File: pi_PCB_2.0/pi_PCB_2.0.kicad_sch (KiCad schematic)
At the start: 7 parts

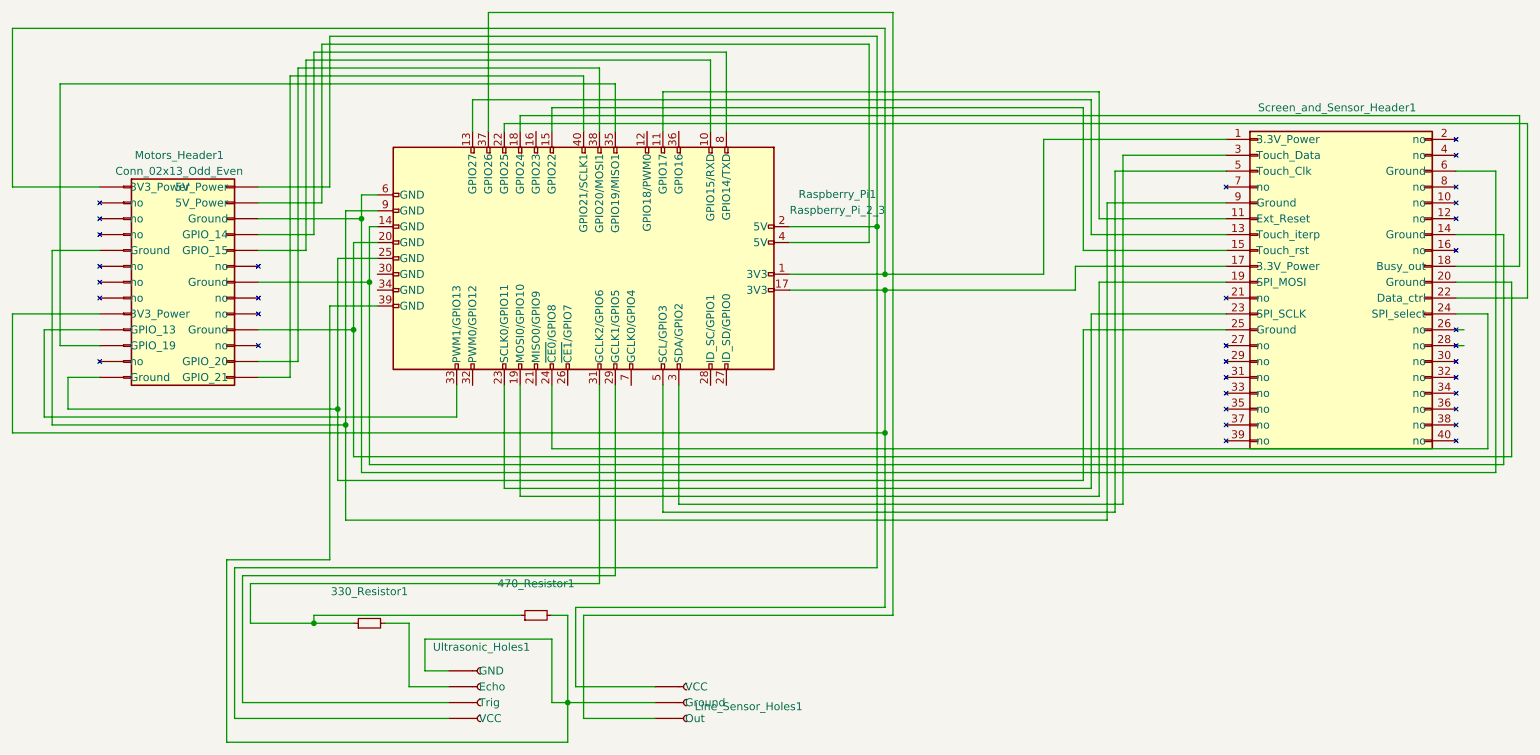
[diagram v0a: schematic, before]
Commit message: PCB Final?
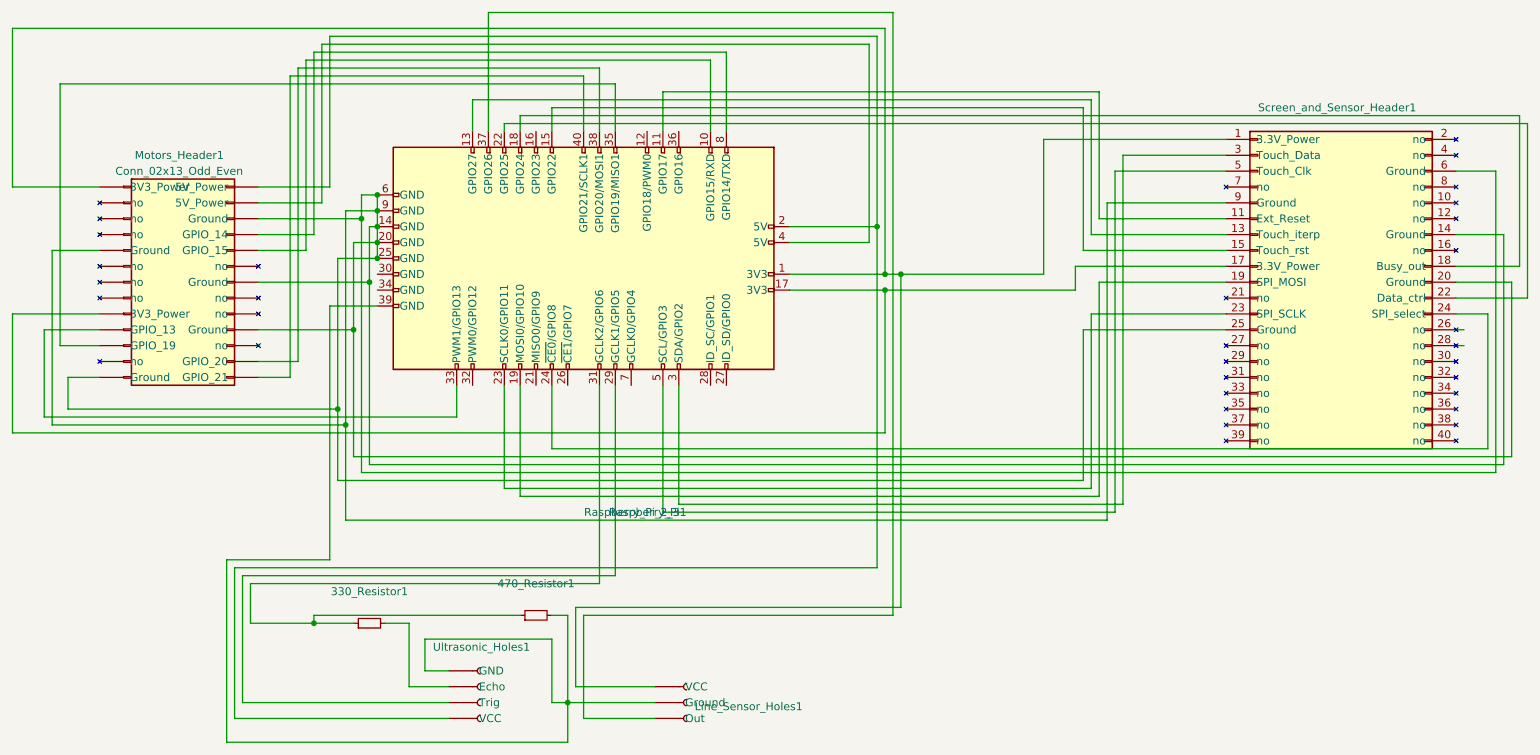
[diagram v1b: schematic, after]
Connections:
- net at Motors_Header1.1 (3V3_Power), Raspberry_Pi1.1 (3V3), Screen_and_Sensor_Header1.1 (3.3V_Power): now also Line_Sensor_Holes1.1 (VCC)
- net at Motors_Header1.14 (Ground), Raspberry_Pi1.14 (GND), Screen_and_Sensor_Header1.14 (Ground): now also Motors_Header1.20 (Ground), Motors_Header1.25 (Ground), Motors_Header1.6 (Ground), Motors_Header1.9 (Ground), Raspberry_Pi1.20 (GND), Raspberry_Pi1.25 (GND), Raspberry_Pi1.6 (GND), Raspberry_Pi1.9 (GND), Screen_and_Sensor_Header1.20 (Ground), Screen_and_Sensor_Header1.25 (Ground), Screen_and_Sensor_Header1.6 (Ground), Screen_and_Sensor_Header1.9 (Ground)
- net at Motors_Header1.17 (3V3_Power), Raspberry_Pi1.17 (3V3), Screen_and_Sensor_Header1.17 (3.3V_Power): no longer Line_Sensor_Holes1.1 (VCC)
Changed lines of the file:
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@@
   (junction (at 163.83 95.25) (diameter 0) (color 0 0 0 0)
   )
+  (junction (at 83.82 92.71) (diameter 0) (color 0 0 0 0)
+  )
   (junction (at 165.1 102.87) (diameter 0) (color 0 0 0 0)
   )
-  (junction (at 165.1 128.27) (diameter 0) (color 0 0 0 0)
-  )
   (junction (at 77.47 124.46) (diameter 0) (color 0 0 0 0)
   )
+  (junction (at 83.82 95.25) (diameter 0) (color 0 0 0 0)
+  )
+  (junction (at 83.82 97.79) (diameter 0) (color 0 0 0 0)
+  )
+  (junction (at 83.82 90.17) (diameter 0) (color 0 0 0 0)
+  )
   (junction (at 82.55 104.14) (diameter 0) (color 0 0 0 0)
   )
@@
   (junction (at 80.01 111.76) (diameter 0) (color 0 0 0 0)
   )
+  (junction (at 83.82 100.33) (diameter 0) (color 0 0 0 0)
+  )
   (junction (at 73.66 158.75) (diameter 0) (color 0 0 0 0)
   )
@@
   (junction (at 78.74 127) (diameter 0) (color 0 0 0 0)
   )
+  (junction (at 167.64 102.87) (diameter 0) (color 0 0 0 0)
+  )
   (junction (at 81.28 93.98) (diameter 0) (color 0 0 0 0)
   )
@@
     (stroke (width 0) (type default))
   )
-  (wire (pts (xy 165.1 128.27) (xy 165.1 156.21))
-    (stroke (width 0) (type default))
-  )
   (wire (pts (xy 82.55 133.35) (xy 82.55 104.14))
     (stroke (width 0) (type default))
@@
     (stroke (width 0) (type default))
   )
-  (wire (pts (xy 115.57 156.21) (xy 165.1 156.21))
-    (stroke (width 0) (type default))
-  )
   (wire (pts (xy 137.16 68.58) (xy 72.39 68.58))
     (stroke (width 0) (type default))
   )
+  (wire (pts (xy 83.82 92.71) (xy 83.82 95.25))
+    (stroke (width 0) (type default))
+  )
   (wire (pts (xy 31.75 127) (xy 31.75 99.06))
     (stroke (width 0) (type default))
@@
     (stroke (width 0) (type default))
   )
-  (wire (pts (xy 190.5 102.87) (xy 165.1 102.87))
+  (wire (pts (xy 190.5 102.87) (xy 167.64 102.87))
     (stroke (width 0) (type default))
   )
@@
     (stroke (width 0) (type default))
   )
+  (wire (pts (xy 115.57 156.21) (xy 167.64 156.21))
+    (stroke (width 0) (type default))
+  )
   (wire (pts (xy 63.5 158.75) (xy 73.66 158.75))
     (stroke (width 0) (type default))
@@
     (stroke (width 0) (type default))
   )
-  (wire (pts (xy 82.55 104.14) (xy 82.55 95.25))
+  (wire (pts (xy 82.55 95.25) (xy 82.55 104.14))
     (stroke (width 0) (type default))
   )
@@
     (stroke (width 0) (type default))
   )
+  (wire (pts (xy 83.82 95.25) (xy 83.82 97.79))
+    (stroke (width 0) (type default))
+  )
   (wire (pts (xy 104.14 78.74) (xy 104.14 80.01))
     (stroke (width 0) (type default))
@@
     (stroke (width 0) (type default))
   )
+  (wire (pts (xy 167.64 102.87) (xy 167.64 156.21))
+    (stroke (width 0) (type default))
+  )
+  (wire (pts (xy 167.64 102.87) (xy 165.1 102.87))
+    (stroke (width 0) (type default))
+  )
   (wire (pts (xy 256.54 96.52) (xy 264.16 96.52))
     (stroke (width 0) (type default))
@@
     (stroke (width 0) (type default))
   )
+  (wire (pts (xy 83.82 90.17) (xy 83.82 92.71))
+    (stroke (width 0) (type default))
+  )
   (wire (pts (xy 201.93 140.97) (xy 129.54 140.97))
     (stroke (width 0) (type default))
@@
   )
   (wire (pts (xy 69.85 71.12) (xy 69.85 119.38))
+    (stroke (width 0) (type default))
+  )
+  (wire (pts (xy 83.82 97.79) (xy 83.82 100.33))
     (stroke (width 0) (type default))
   )
@@
   (symbol (lib_id "Connector:Raspberry_Pi_2_3") (at 116.84 100.33 270) (unit 1)
     (in_bom yes) (on_board yes) (dnp no) (fields_autoplaced)
-    (property "Reference" "Raspberry_Pi1" (at 157.48 90.0683 90)
+    (property "Reference" "Raspberry_Pi1" (at 127.1017 140.97 90)
       (effects (font (size 1.27 1.27)))
     )
-    (property "Value" "Raspberry_Pi_2_3" (at 157.48 92.6083 90)
+    (property "Value" "Raspberry_Pi_2_3" (at 124.5617 140.97 90)
       (effects (font (size 1.27 1.27)))
     )

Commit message: Final 3
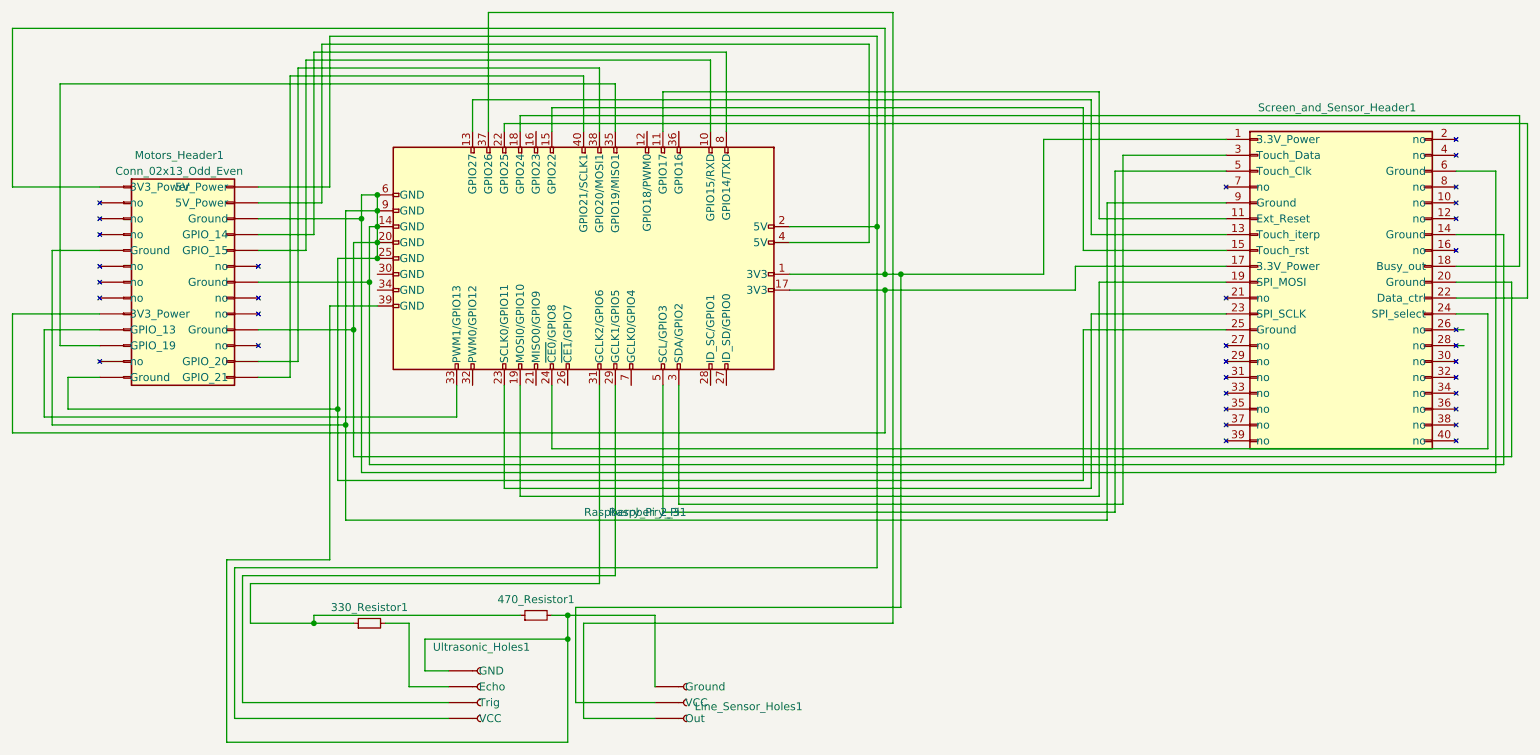
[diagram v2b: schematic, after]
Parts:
- 330_Resistor1, 470_Resistor1: footprint Resistor_THT:R_Axial_DIN0204_L3.6mm_D1.6mm_P1.90mm_Vertical -> Resistor_THT:R_Axial_DIN0207_L6.3mm_D2.5mm_P10.16mm_Horizontal
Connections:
- net at Motors_Header1.1 (3V3_Power), Raspberry_Pi1.1 (3V3), Screen_and_Sensor_Header1.1 (3.3V_Power): now also Line_Sensor_Holes1.2 (VCC); no longer Line_Sensor_Holes1.1 (VCC)
- net at 470_Resistor1.2, Raspberry_Pi1.39 (GND), Ultrasonic_Holes1.1 (GND): now also Line_Sensor_Holes1.1 (Ground); no longer Line_Sensor_Holes1.2 (Ground)
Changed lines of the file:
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@@
 (kicad_sch (version 20230121) (generator eeschema)
   (paper "A4")
+  (junction (at 114.3 157.48) (diameter 0) (color 0 0 0 0)
+  )
   (junction (at 163.83 95.25) (diameter 0) (color 0 0 0 0)
   )
@@
   (junction (at 80.01 111.76) (diameter 0) (color 0 0 0 0)
   )
+  (junction (at 114.3 161.29) (diameter 0) (color 0 0 0 0)
+  )
   (junction (at 83.82 100.33) (diameter 0) (color 0 0 0 0)
   )
   (junction (at 73.66 158.75) (diameter 0) (color 0 0 0 0)
   )
-  (junction (at 114.3 171.45) (diameter 0) (color 0 0 0 0)
-  )
   (junction (at 78.74 127) (diameter 0) (color 0 0 0 0)
   )
@@
     (stroke (width 0) (type default))
   )
-  (wire (pts (xy 111.76 171.45) (xy 114.3 171.45))
-    (stroke (width 0) (type default))
-  )
   (wire (pts (xy 199.39 138.43) (xy 199.39 104.14))
     (stroke (width 0) (type default))
@@
     (stroke (width 0) (type default))
   )
-  (wire (pts (xy 115.57 168.91) (xy 128.27 168.91))
-    (stroke (width 0) (type default))
-  )
   (wire (pts (xy 30.48 111.76) (xy 39.37 111.76))
     (stroke (width 0) (type default))
@@
     (stroke (width 0) (type default))
   )
-  (wire (pts (xy 166.37 60.96) (xy 166.37 157.48))
+  (wire (pts (xy 166.37 60.96) (xy 166.37 158.75))
     (stroke (width 0) (type default))
   )
@@
     (stroke (width 0) (type default))
   )
+  (wire (pts (xy 114.3 161.29) (xy 114.3 177.8))
+    (stroke (width 0) (type default))
+  )
   (wire (pts (xy 195.58 101.6) (xy 195.58 105.41))
     (stroke (width 0) (type default))
@@
     (stroke (width 0) (type default))
   )
-  (wire (pts (xy 111.76 157.48) (xy 114.3 157.48))
-    (stroke (width 0) (type default))
-  )
   (wire (pts (xy 106.68 138.43) (xy 199.39 138.43))
     (stroke (width 0) (type default))
@@
     (stroke (width 0) (type default))
   )
-  (wire (pts (xy 115.57 156.21) (xy 115.57 168.91))
+  (wire (pts (xy 115.57 156.21) (xy 115.57 171.45))
     (stroke (width 0) (type default))
   )
@@
     (stroke (width 0) (type default))
   )
-  (wire (pts (xy 114.3 171.45) (xy 128.27 171.45))
-    (stroke (width 0) (type default))
-  )
   (wire (pts (xy 63.5 152.4) (xy 63.5 158.75))
     (stroke (width 0) (type default))
@@
     (stroke (width 0) (type default))
   )
-  (wire (pts (xy 91.44 161.29) (xy 111.76 161.29))
+  (wire (pts (xy 91.44 161.29) (xy 114.3 161.29))
     (stroke (width 0) (type default))
   )
@@
     (stroke (width 0) (type default))
   )
-  (wire (pts (xy 114.3 171.45) (xy 114.3 177.8))
-    (stroke (width 0) (type default))
-  )
   (wire (pts (xy 256.54 106.68) (xy 267.97 106.68))
     (stroke (width 0) (type default))
@@
     (stroke (width 0) (type default))
   )
-  (wire (pts (xy 166.37 157.48) (xy 116.84 157.48))
+  (wire (pts (xy 166.37 158.75) (xy 116.84 158.75))
     (stroke (width 0) (type default))
   )
@@
     (stroke (width 0) (type default))
   )
-  (wire (pts (xy 111.76 161.29) (xy 111.76 171.45))
+  (wire (pts (xy 114.3 157.48) (xy 114.3 161.29))
+    (stroke (width 0) (type default))
+  )
+  (wire (pts (xy 114.3 157.48) (xy 111.76 157.48))
+    (stroke (width 0) (type default))
+  )
+  (wire (pts (xy 128.27 171.45) (xy 115.57 171.45))
     (stroke (width 0) (type default))
   )
@@
     (stroke (width 0) (type default))
   )
+  (wire (pts (xy 128.27 157.48) (xy 128.27 168.91))
+    (stroke (width 0) (type default))
+  )
   (wire (pts (xy 121.92 120.65) (xy 121.92 151.13))
     (stroke (width 0) (type default))
@@
     (stroke (width 0) (type default))
   )
-  (wire (pts (xy 114.3 157.48) (xy 114.3 171.45))
-    (stroke (width 0) (type default))
-  )
   (wire (pts (xy 25.4 63.5) (xy 25.4 88.9))
     (stroke (width 0) (type default))
@@
     (stroke (width 0) (type default))
   )
-  (wire (pts (xy 116.84 157.48) (xy 116.84 173.99))
+  (wire (pts (xy 116.84 158.75) (xy 116.84 173.99))
     (stroke (width 0) (type default))
   )
@@
   )
   (wire (pts (xy 33.02 72.39) (xy 121.92 72.39))
+    (stroke (width 0) (type default))
+  )
+  (wire (pts (xy 114.3 157.48) (xy 128.27 157.48))
     (stroke (width 0) (type default))
   )
@@
   (symbol (lib_id "Device:R_Small") (at 109.22 157.48 90) (unit 1)
     (in_bom yes) (on_board yes) (dnp no) (fields_autoplaced)
-    (property "Reference" "470_Resistor1" (at 109.22 152.4 90)
+    (property "Reference" "470_Resistor1" (at 109.22 154.94 90)
       (effects (font (size 1.27 1.27)))
     )
@@
       (effects (font (size 1.27 1.27)) hide)
     )
-    (property "Footprint" "Resistor_THT:R_Axial_DIN0204_L3.6mm_D1.6mm_P1.90mm_Vertical" (at 109.22 157.48 0)
+    (property "Footprint" "Resistor_THT:R_Axial_DIN0207_L6.3mm_D2.5mm_P10.16mm_Horizontal" (at 109.22 157.48 0)
       (effects (font (size 1.27 1.27)) hide)
     )
@@
   (symbol (lib_id "Device:R_Small") (at 82.55 158.75 90) (unit 1)
     (in_bom yes) (on_board yes) (dnp no) (fields_autoplaced)
-    (property "Reference" "330_Resistor1" (at 82.55 153.67 90)
+    (property "Reference" "330_Resistor1" (at 82.55 156.21 90)
       (effects (font (size 1.27 1.27)))
     )
@@
       (effects (font (size 1.27 1.27)) hide)
     )
-    (property "Footprint" "Resistor_THT:R_Axial_DIN0204_L3.6mm_D1.6mm_P1.90mm_Vertical" (at 82.55 158.75 0)
-      (effects (font (size 1.27 1.27)) hide)
-    )
+    (property "Footprint" "Resistor_THT:R_Axial_DIN0207_L6.3mm_D2.5mm_P10.16mm_Horizontal" (at 82.55 158.75 0)
+      (effects (font (size 1.27 1.27)) hide)
+    )
